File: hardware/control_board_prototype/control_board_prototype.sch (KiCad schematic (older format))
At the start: 76 parts, among them J1 Conn_01x17_Male, J10 Conn_02x06_Odd_Even, J11 Conn_02x10_Odd_Even, J12 Conn_02x04_Odd_Even, J2 Conn_01x15_Male, J3 Conn_01x02_Male, J4 Conn_02x10_Odd_Even, J5 Conn_02x10_Odd_Even, J6 Conn_02x10_Odd_Even, J7 Conn_02x04_Odd_Even, J8 Conn_02x06_Odd_Even, J9 Conn_02x04_Odd_Even, U1 LM317, U2 LM358, U3 TLE2426xLP, U4 BU2505FV, U5 BU2505FV

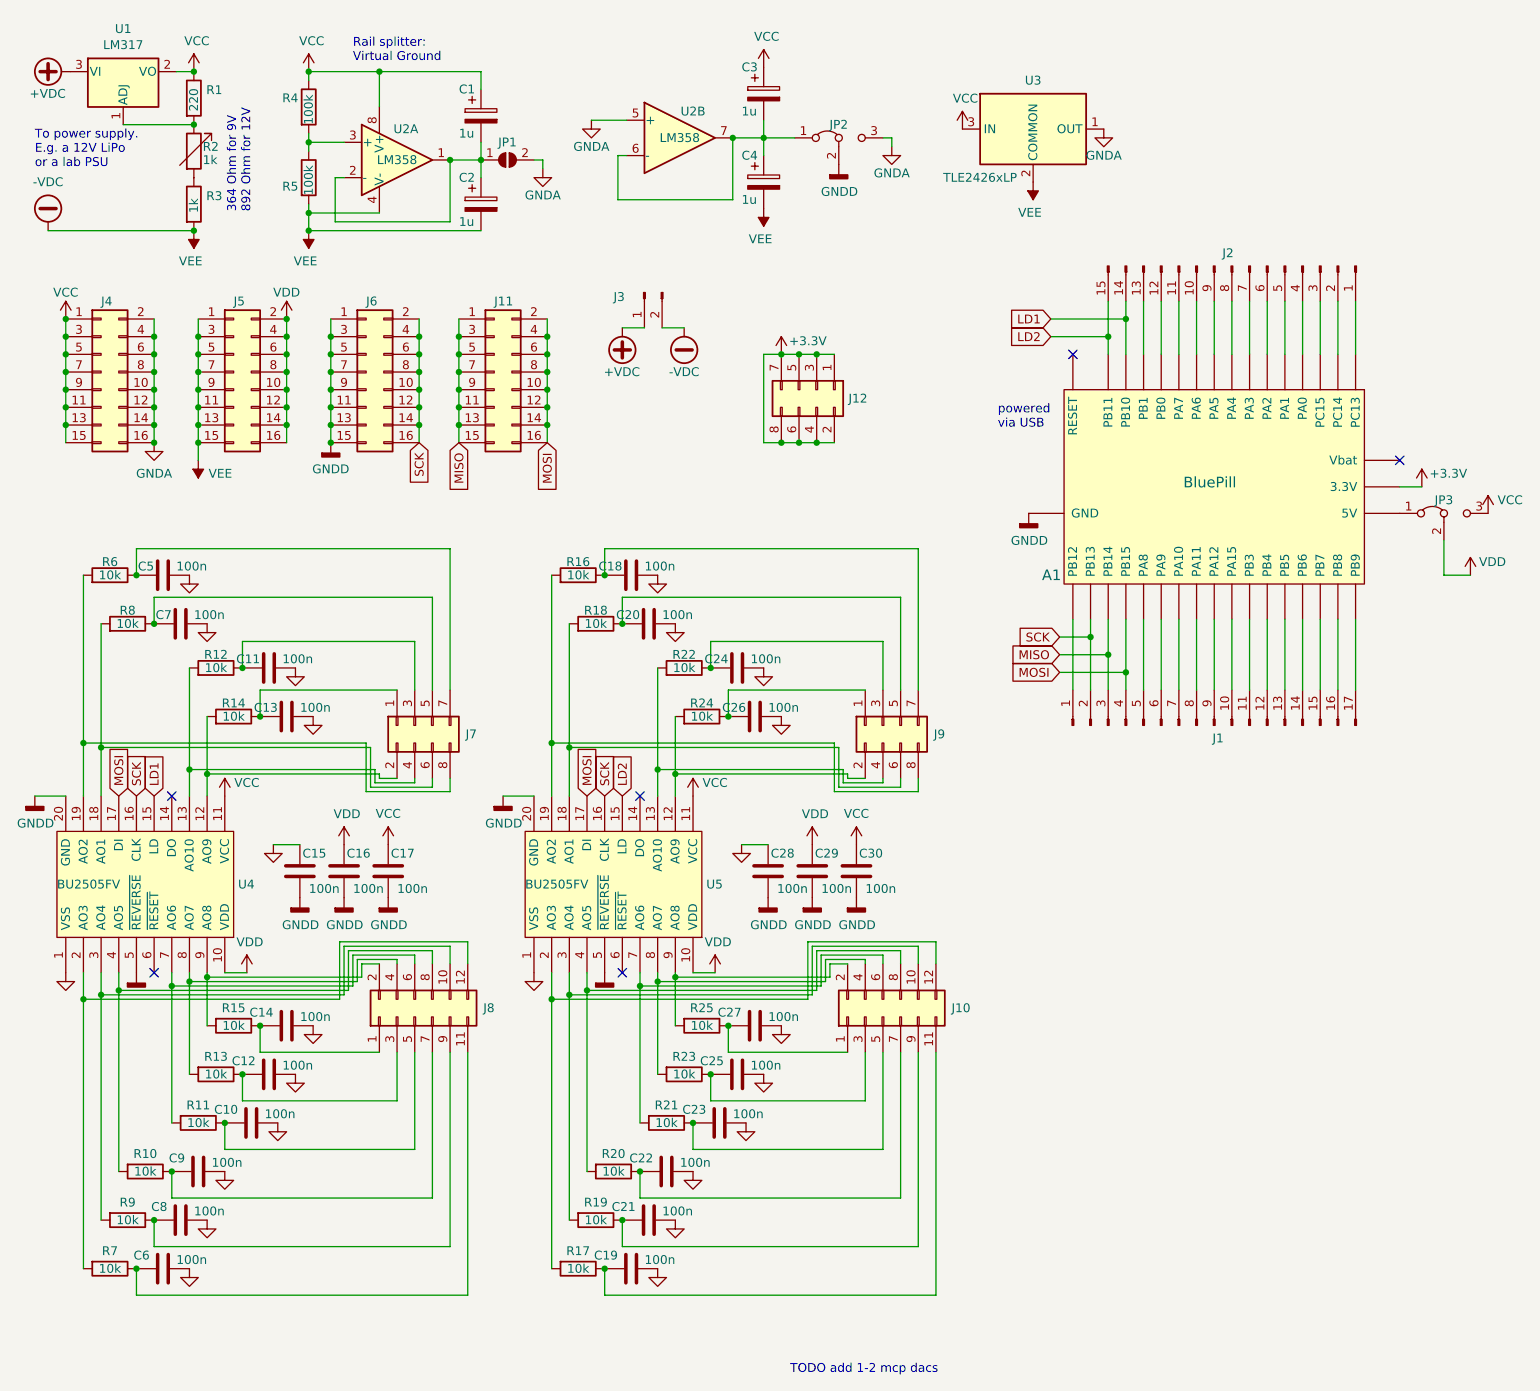
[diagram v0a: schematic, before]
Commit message: reality update for the control board:
- reduce R4/R5 from 100k to 2.2k
- capacitors across R5 and U1
- protection diode for U1
- source termination resistor for SCK signal
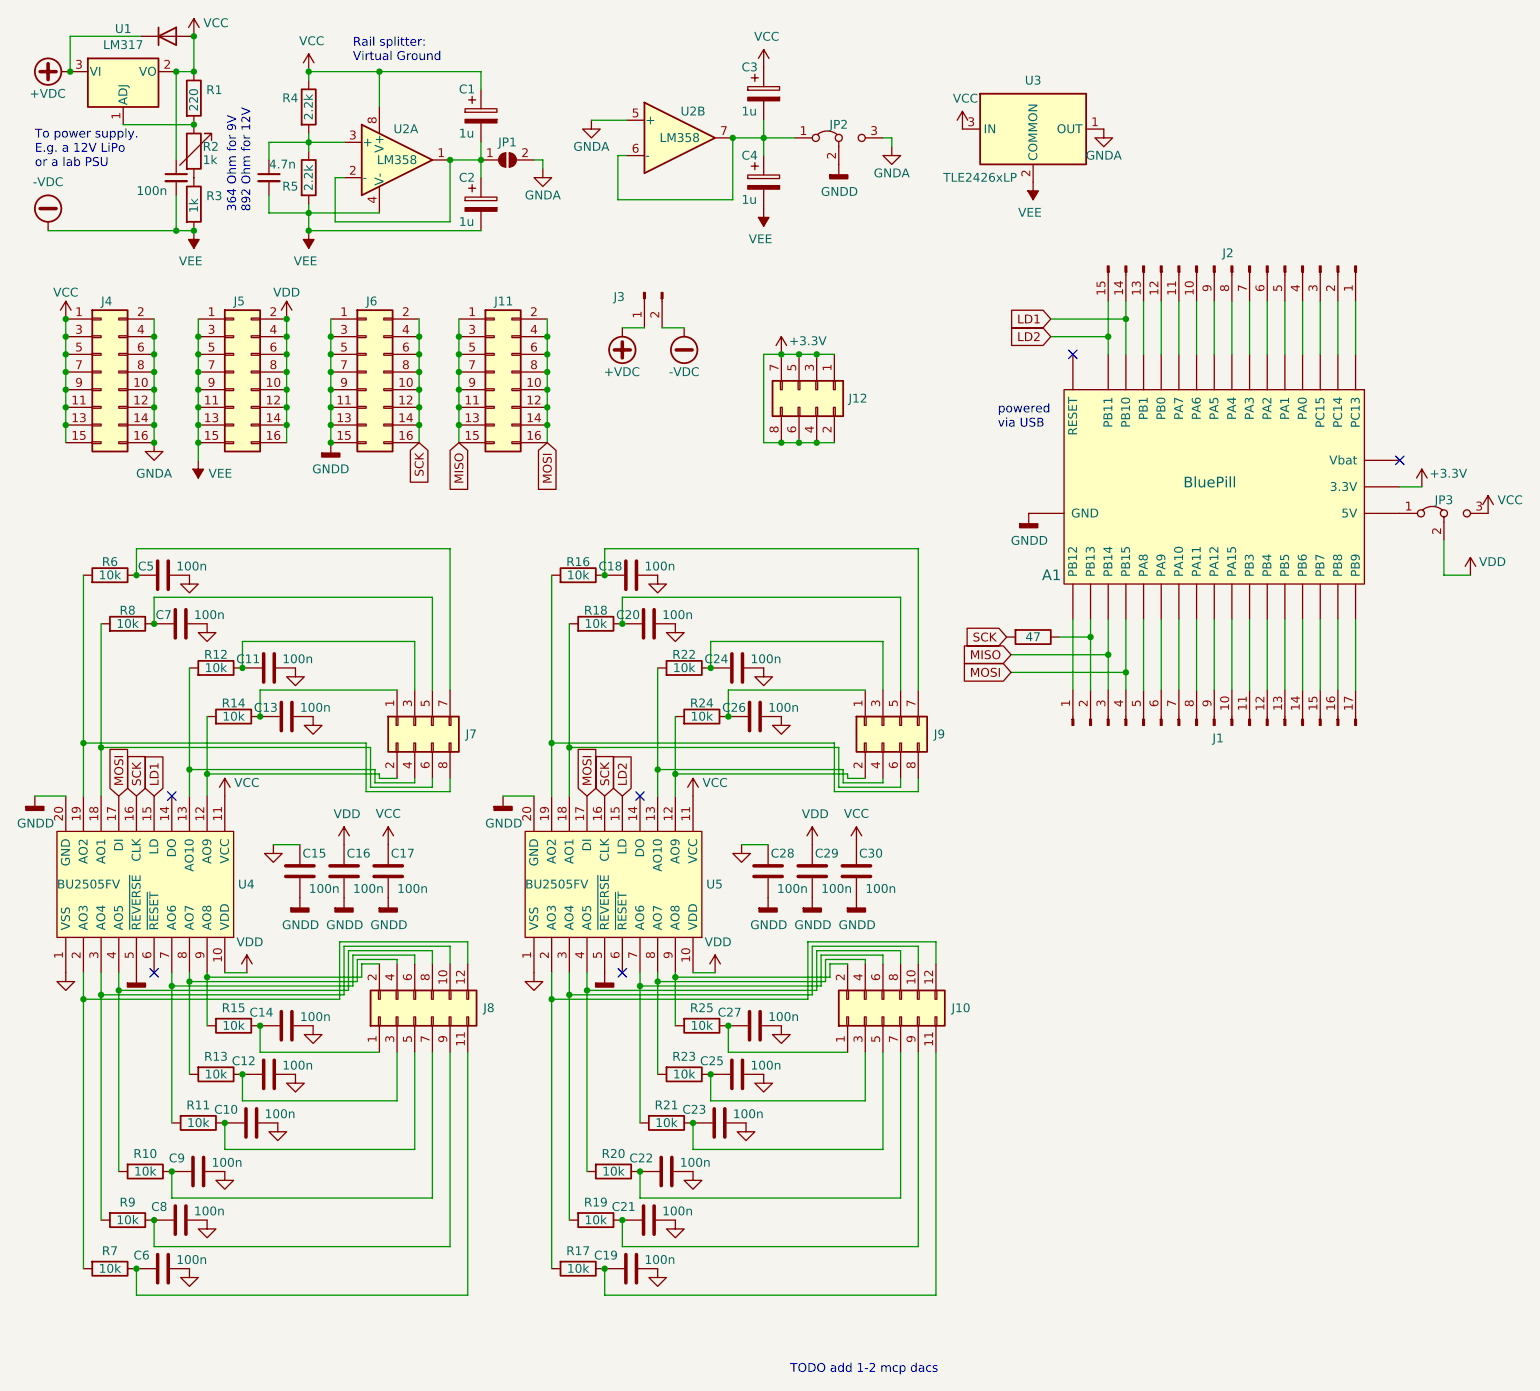
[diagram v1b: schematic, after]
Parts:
- added C?: 4.7n, symbol Device:C_Small
- added C?: 100n, symbol Device:C_Small
- added D?: D, symbol Device:D
- added R?: 47, symbol Device:R
- R4, R5: value 100k -> 2.2k
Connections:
- net +VDC: now also D?.1 (K)
- net -VDC: now also C?.2, C?.2
- net SCK: now also R?.2; no longer A1.PB13, J1.2 (Pin_2)
- net VCC: now also C?.1, D?.2 (A)
- net at R4.2, R5.1, U2.3 (+): now also C?.1
- new net: A1.PB13, J1.2 (Pin_2), R?.1
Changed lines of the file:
@@
 EESchema Schematic File Version 4
-LIBS:control_board_prototype-cache
 EELAYER 30 0
 EELAYER END
@@
 LD1
 Wire Wire Line
-	6375 4225 6750 4225
+	6100 4225 6750 4225
 Wire Wire Line
 	6650 4125 6650 3925
 Wire Wire Line
-	6375 4125 6650 4125
-Text GLabel 6375 4125 0    50   Input ~ 0
+	6100 4125 6650 4125
+Text GLabel 6100 4125 0    50   Input ~ 0
 MISO
 Wire Wire Line
@@
 L power:VCC #PWR03
 U 1 1 5FA03DB1
-P 1475 825
-F 0 "#PWR03" H 1475 675 50  0001 C CNN
-F 1 "VCC" H 1492 998 50  0000 C CNN
-F 2 "" H 1475 825 50  0001 C CNN
-F 3 "" H 1475 825 50  0001 C CNN
-	1    1475 825
+P 1475 625
+F 0 "#PWR03" H 1475 475 50  0001 C CNN
+F 1 "VCC" H 1600 700 50  0000 C CNN
+F 2 "" H 1475 625 50  0001 C CNN
+F 3 "" H 1475 625 50  0001 C CNN
+	1    1475 625
 	1    0    0    -1
 $EndComp
@@
 	1    0    0    -1
 $EndComp
-Text GLabel 6375 4025 0    50   Input ~ 0
-SCK
-Text GLabel 6375 4225 0    50   Input ~ 0
+Text GLabel 6100 4225 0    50   Input ~ 0
 MOSI
 Wire Wire Line
@@
 Rail splitter:\nVirtual Ground
 Connection ~ 2125 1225
-Wire Wire Line
-	2125 1225 2325 1225
 $Comp
 L Device:CP C1
@@
 Connection ~ 2125 825
 Wire Wire Line
-	2125 825  2525 825
-Wire Wire Line
 	2125 1225 2125 1275
 $Comp
@@
 P 2125 1425
 F 0 "R5" H 1975 1375 50  0000 L CNN
-F 1 "100k" V 2125 1325 50  0000 L CNN
+F 1 "2.2k" V 2125 1350 50  0000 L CNN
 F 2 "Resistor_SMD:R_0805_2012Metric_Pad1.15x1.40mm_HandSolder" V 2055 1425 50  0001 C CNN
 F 3 "~" H 2125 1425 50  0001 C CNN
@@
 P 2125 1025
 F 0 "R4" H 1975 1075 50  0000 L CNN
-F 1 "100k" V 2125 925 50  0000 L CNN
+F 1 "2.2k" V 2125 950 50  0000 L CNN
 F 2 "Resistor_SMD:R_0805_2012Metric_Pad1.15x1.40mm_HandSolder" V 2055 1025 50  0001 C CNN
 F 3 "~" H 2125 1025 50  0001 C CNN
@@
 To power supply.\nE.g. a 12V LiPo\nor a lab PSU
 Wire Wire Line
-	650  1725 1475 1725
+	650  1725 1375 1725
 $Comp
 L power:-VDC #PWR01
@@
 Wire Wire Line
 	5000 2925 5100 2925
+$Comp
+L Device:C_Small C?
+U 1 1 600A4DC0
+P 1900 1425
+F 0 "C?" H 1925 1575 50  0001 L CNN
+F 1 "4.7n" H 1900 1500 50  0000 L CNN
+F 2 "" H 1900 1425 50  0001 C CNN
+F 3 "~" H 1900 1425 50  0001 C CNN
+	1    1900 1425
+	1    0    0    -1
+$EndComp
+$Comp
+L Device:D D?
+U 1 1 600EF493
+P 1325 625
+F 0 "D?" H 1325 842 50  0001 C CNN
+F 1 "D" H 1325 725 50  0001 C CNN
+F 2 "" H 1325 625 50  0001 C CNN
+F 3 "~" H 1325 625 50  0001 C CNN
+	1    1325 625
+	1    0    0    -1
+$EndComp
+Wire Wire Line
+	1475 625  1475 825
+Connection ~ 1475 625
+Wire Wire Line
+	1175 625  775  625
+Wire Wire Line
+	775  625  775  825
+Connection ~ 775  825
+$Comp
+L Device:C_Small C?
+U 1 1 6013C8D9
+P 1375 1425
+F 0 "C?" H 1400 1575 50  0001 L CNN
+F 1 "100n" H 1150 1350 50  0000 L CNN
+F 2 "" H 1375 1425 50  0001 C CNN
+F 3 "~" H 1375 1425 50  0001 C CNN
+	1    1375 1425
+	1    0    0    -1
+$EndComp
+Connection ~ 1375 825
+Wire Wire Line
+	1375 1525 1375 1725
+Connection ~ 1375 1725
+Wire Wire Line
+	1375 1725 1475 1725
+Wire Wire Line
+	1375 825  1375 1325
+Text GLabel 6075 4025 0    50   Input ~ 0
+SCK
+$Comp
+L Device:R R?
+U 1 1 6020E31A
+P 6225 4025
+F 0 "R?" V 6125 4050 50  0001 C CNN
+F 1 "47" V 6225 4025 50  0000 C CNN
+F 2 "" V 6155 4025 50  0001 C CNN
+F 3 "~" H 6225 4025 50  0001 C CNN
+	1    6225 4025
+	0    1    1    0
+$EndComp
+Wire Wire Line
+	2125 825  2525 825
+Wire Wire Line
+	2125 1225 2325 1225
+Wire Wire Line
+	2125 1225 1900 1225
+Wire Wire Line
+	1900 1225 1900 1325
+Wire Wire Line
+	1900 1525 1900 1625
+Wire Wire Line
+	1900 1625 2125 1625
 $EndSCHEMATC
